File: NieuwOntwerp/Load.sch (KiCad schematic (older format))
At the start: 81 parts, among them J1 USB_C_Receptacle_USB2.0, J2 Conn_01x02, Q1 Si2306, Q2 4809NG, Q3 IRF840, Q4 IRF840, Q5 IRF840, U1 ESP12E, U2 FT231XQ, U3 LM358, U4 MCP4725A0, U5 LM358, U6 

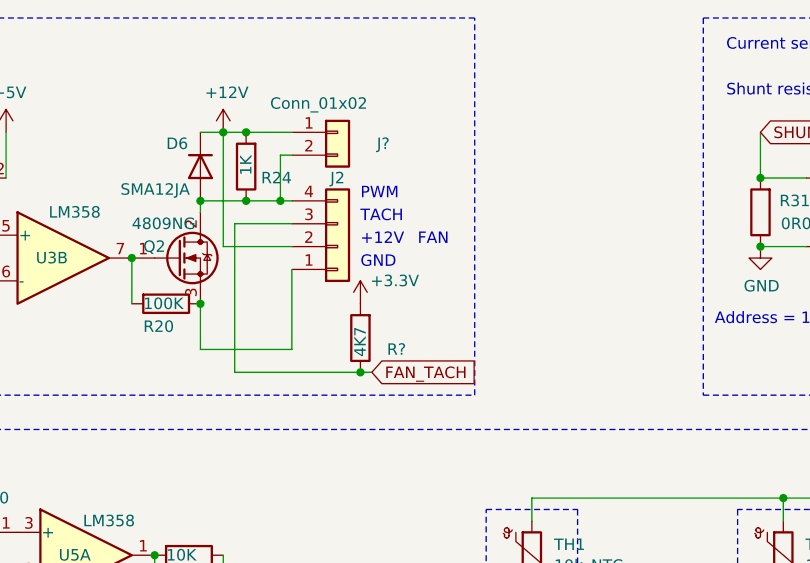
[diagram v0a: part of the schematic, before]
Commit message: 2021-05-14_01
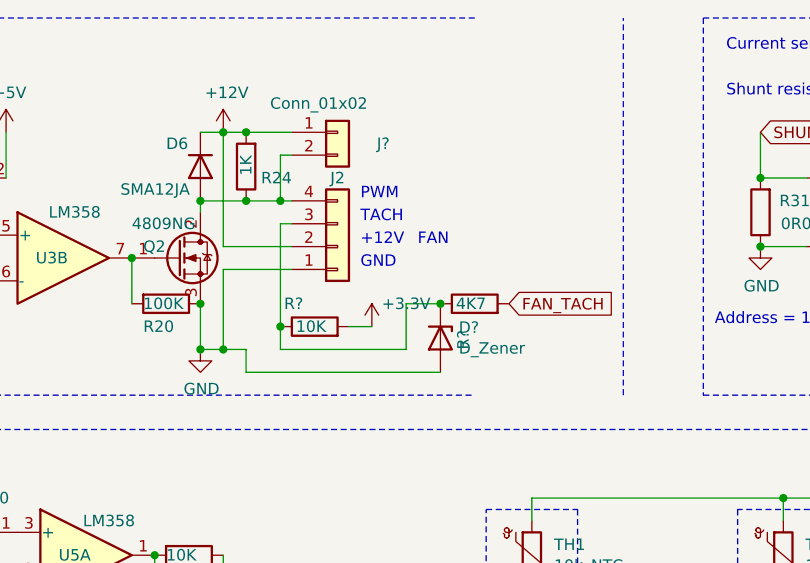
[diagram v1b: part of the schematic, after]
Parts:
- added D?: D_Zener, symbol Device:D_Zener
- added R?: 4K7, Resistor_SMD:R_0603_1608Metric, symbol Device:R
- R?: value 4K7 -> 10K
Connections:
- net FAN_TACH: now also R?.2; no longer J2.3 (Pin_3), R?.1
- net GND: now also J2.1 (Pin_1), Q2.3 (S), R20.1, D?.2 (A)
- new net: D?.1 (K), J2.3 (Pin_3), R?.1, R?.1
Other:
- moved on the sheet: R?
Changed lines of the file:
@@
 	6600 1450 6800 1450
 Connection ~ 6600 1450
-Text GLabel 7350 2200 2    50   Input ~ 0
+Text GLabel 7950 1900 2    50   Input ~ 0
 FAN_TACH
 $Comp
@@
 	4400 2300 7800 2300
 Wire Notes Line
-	7800 2300 7800 650
+	8450 2300 8450 650
 Wire Notes Line
 	7800 650  4400 650
@@
 Connection ~ 6800 1450
 Wire Wire Line
-	7000 1750 7000 2100
-Wire Wire Line
 	4850 1600 5450 1600
 Connection ~ 5450 1600
@@
 	2400 3650 2400 3700
 Wire Wire Line
-	6600 2100 7000 2100
+	6600 2100 6700 2100
 $Comp
 L Device:Q_NMOS_GSD Q?
@@
 L Device:R R?
 U 1 1 60A70C52
-P 7300 2050
-F 0 "R?" H 7100 2100 50  0000 L CNN
-F 1 "4K7" V 7300 2000 50  0000 L CNN
-F 2 "Resistor_SMD:R_0603_1608Metric" V 7230 2050 50  0001 C CNN
-F 3 "~" H 7300 2050 50  0001 C CNN
-	1    7300 2050
-	-1   0    0    1
+P 7100 2000
+F 0 "R?" V 7200 2050 50  0000 L CNN
+F 1 "10K" V 7100 1950 50  0000 L CNN
+F 2 "Resistor_SMD:R_0603_1608Metric" V 7030 2000 50  0001 C CNN
+F 3 "~" H 7100 2000 50  0001 C CNN
+	1    7100 2000
+	0    -1   -1   0
 $EndComp
 $Comp
 L power:+3.3V #PWR?
 U 1 1 60A70C58
-P 7300 1900
-F 0 "#PWR?" H 7300 1750 50  0001 C CNN
-F 1 "+3.3V" H 7450 2000 50  0000 C CNN
-F 2 "" H 7300 1900 50  0001 C CNN
-F 3 "" H 7300 1900 50  0001 C CNN
-	1    7300 1900
-	1    0    0    -1
-$EndComp
-Wire Wire Line
-	7350 2200 7300 2200
-Wire Wire Line
-	6750 1550 6750 2200
-Connection ~ 7300 2200
-Wire Wire Line
-	7300 2200 6750 2200
+P 7350 2000
+F 0 "#PWR?" H 7350 1850 50  0001 C CNN
+F 1 "+3.3V" H 7500 2100 50  0000 C CNN
+F 2 "" H 7350 2000 50  0001 C CNN
+F 3 "" H 7350 2000 50  0001 C CNN
+	1    7350 2000
+	1    0    0    -1
+$EndComp
 Wire Wire Line
 	6800 1150 7000 1150
 Connection ~ 6800 1150
 Wire Wire Line
-	6750 1550 7000 1550
-Wire Wire Line
 	6950 1450 6950 1250
 Wire Wire Line
@@
 Wire Wire Line
 	6950 1450 7000 1450
+$Comp
+L Device:R R?
+U 1 1 60A04DE5
+P 7800 1900
+F 0 "R?" H 7600 1950 50  0000 L CNN
+F 1 "4K7" V 7800 1850 50  0000 L CNN
+F 2 "Resistor_SMD:R_0603_1608Metric" V 7730 1900 50  0001 C CNN
+F 3 "~" H 7800 1900 50  0001 C CNN
+	1    7800 1900
+	0    -1   -1   0
+$EndComp
+Wire Wire Line
+	7350 2000 7250 2000
+$Comp
+L power:GND #PWR?
+U 1 1 60A47FC5
+P 6600 2100
+F 0 "#PWR?" H 6600 1850 50  0001 C CNN
+F 1 "GND" H 6605 1927 50  0000 C CNN
+F 2 "" H 6600 2100 50  0001 C CNN
+F 3 "" H 6600 2100 50  0001 C CNN
+	1    6600 2100
+	1    0    0    -1
+$EndComp
+Connection ~ 6600 2100
+Wire Wire Line
+	6950 1550 6950 2000
+Wire Wire Line
+	6950 1550 7000 1550
+Wire Wire Line
+	7000 1750 6700 1750
+Wire Wire Line
+	6700 1750 6700 2100
+$Comp
+L Device:D_Zener D?
+U 1 1 60A2F1AD
+P 7650 2050
+F 0 "D?" V 7604 2130 50  0000 L CNN
+F 1 "D_Zener" V 7695 2130 50  0000 L CNN
+F 2 "" H 7650 2050 50  0001 C CNN
+F 3 "~" H 7650 2050 50  0001 C CNN
+	1    7650 2050
+	0    1    1    0
+$EndComp
+Wire Wire Line
+	7650 1900 7500 1900
+Wire Wire Line
+	7500 1900 7500 2100
+Wire Wire Line
+	7500 2100 6950 2100
+Wire Wire Line
+	6950 2100 6950 2000
+Connection ~ 7650 1900
+Connection ~ 6950 2000
+Wire Wire Line
+	6700 2100 6800 2100
+Wire Wire Line
+	6800 2100 6800 2200
+Wire Wire Line
+	6800 2200 7650 2200
+Connection ~ 6700 2100
 $EndSCHEMATC
